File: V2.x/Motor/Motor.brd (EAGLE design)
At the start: 43.2 x 34.3 mm, 48 parts, among them IC1 Atmega 328-P, IC2 MCP2515, IC3 LM340MP-05, Q1 8MHz, Q2 16MHz

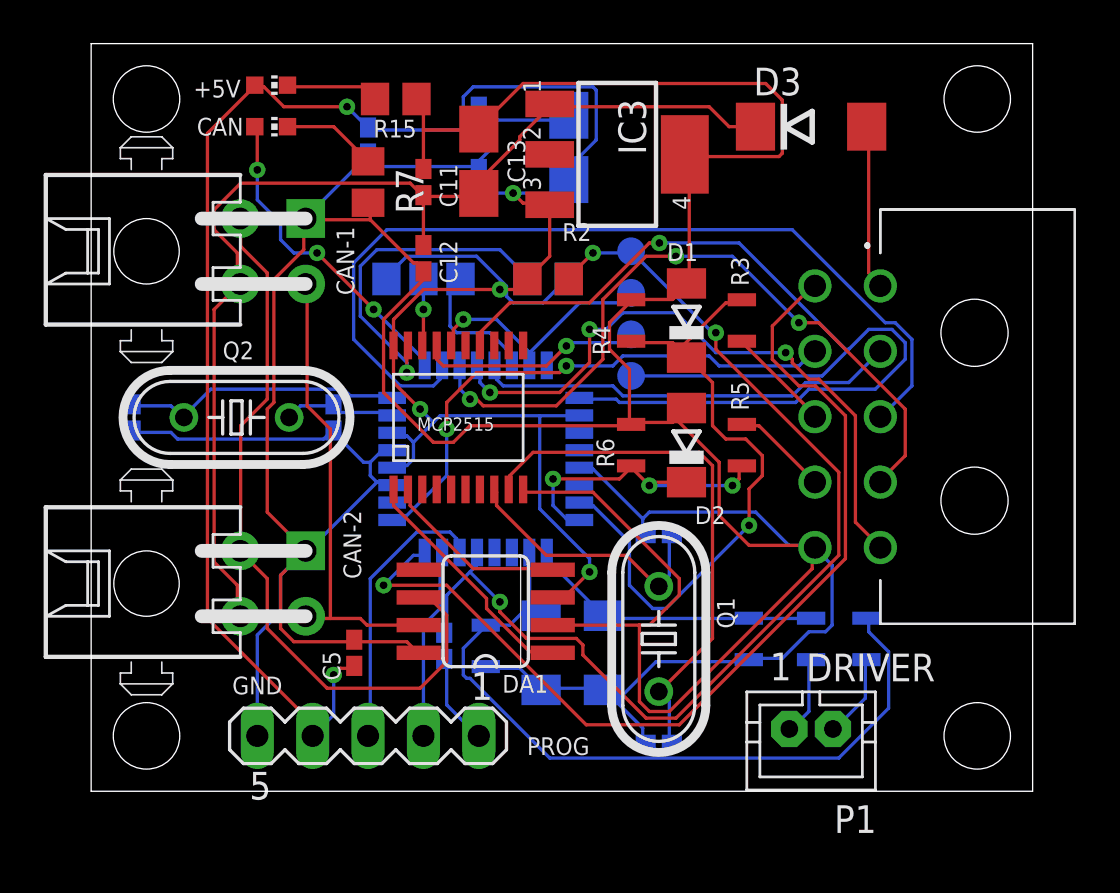
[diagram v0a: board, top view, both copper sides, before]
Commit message: initial
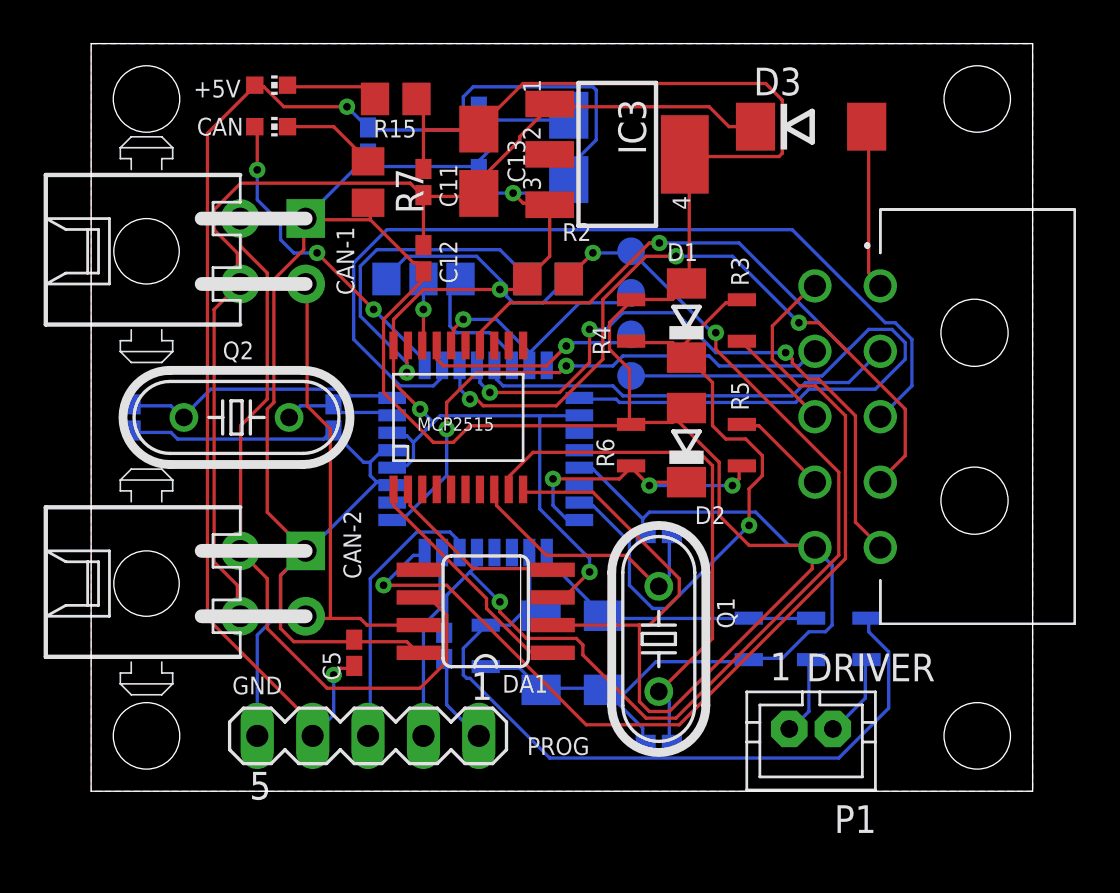
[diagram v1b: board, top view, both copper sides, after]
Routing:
- added copper zone on layer 1, net GND
- added copper zone on layer 16, net GND
